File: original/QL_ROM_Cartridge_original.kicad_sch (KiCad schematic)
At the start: 6 parts, among them IC1 27C128, IC2 27C128, IC3 74LS00, J1 QL_cartridge_ROM

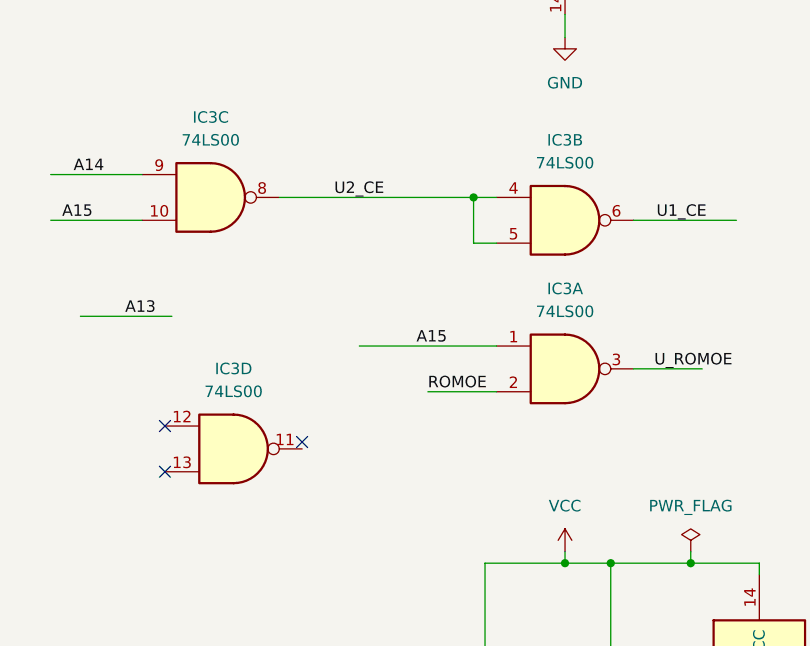
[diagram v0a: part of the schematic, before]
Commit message: update
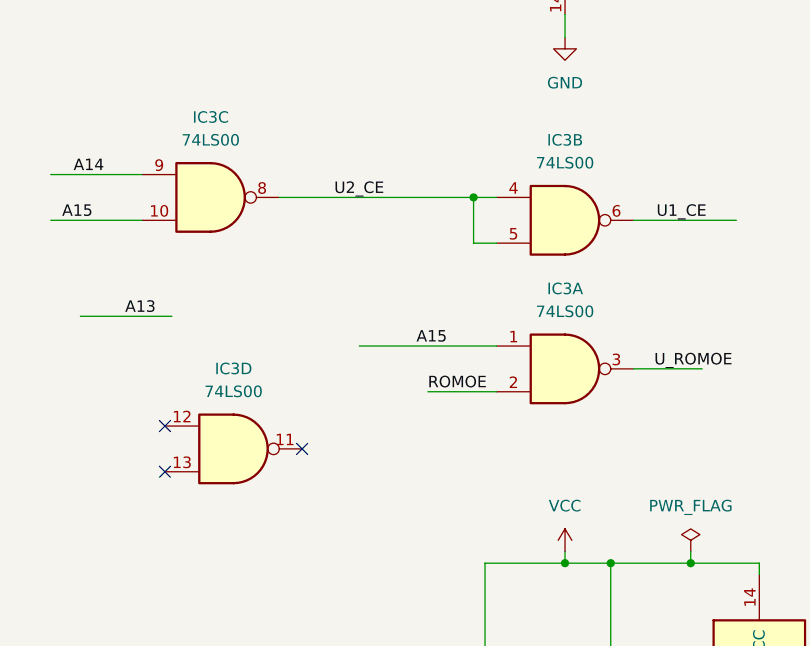
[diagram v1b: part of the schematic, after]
